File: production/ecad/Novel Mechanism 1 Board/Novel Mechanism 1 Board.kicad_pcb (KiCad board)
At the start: 2 copper layers, 39 parts, among them J1 Conn_01x02_Socket, J2 Conn_01x02_Socket, J3 Conn_01x02_Socket, J4 0532611271, U1 ADC081C021CIMM/NOPB, U2 ADC081C021CIMM/NOPB, U3 ADC081C021CIMM/NOPB

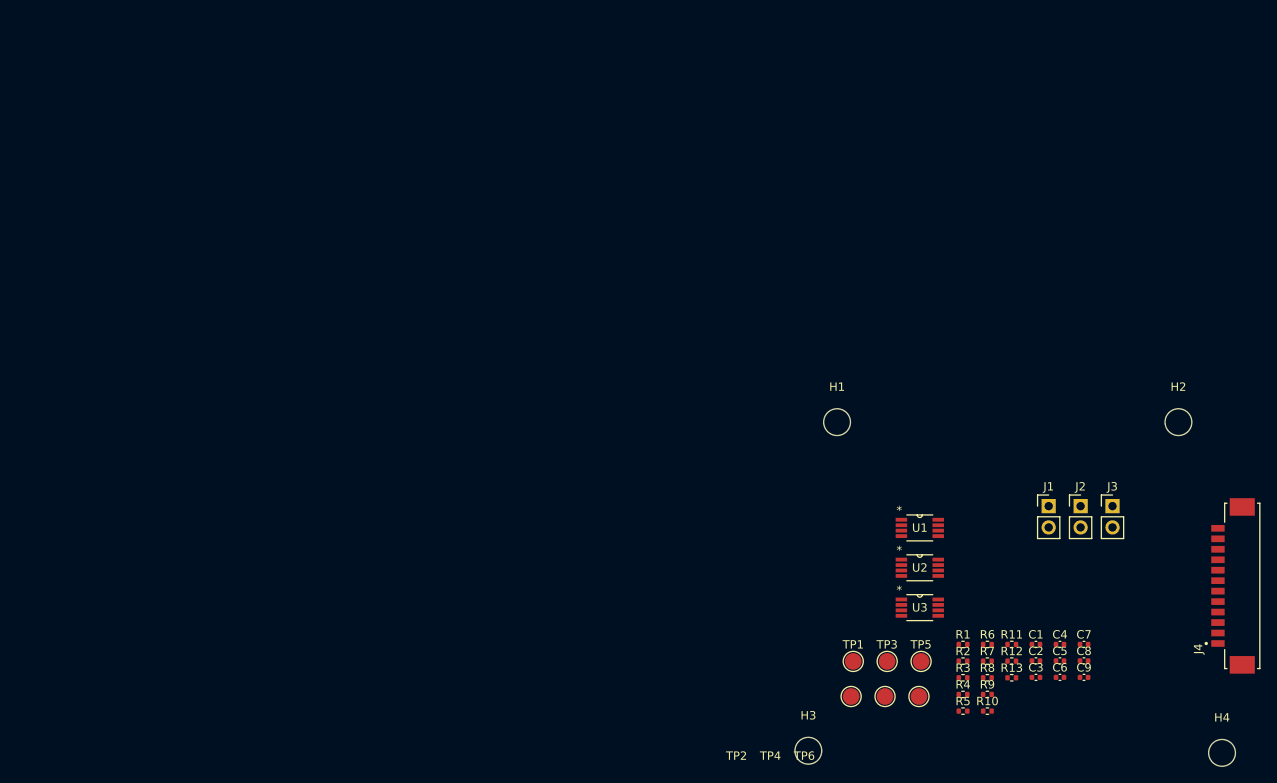
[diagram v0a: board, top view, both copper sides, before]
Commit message: layout
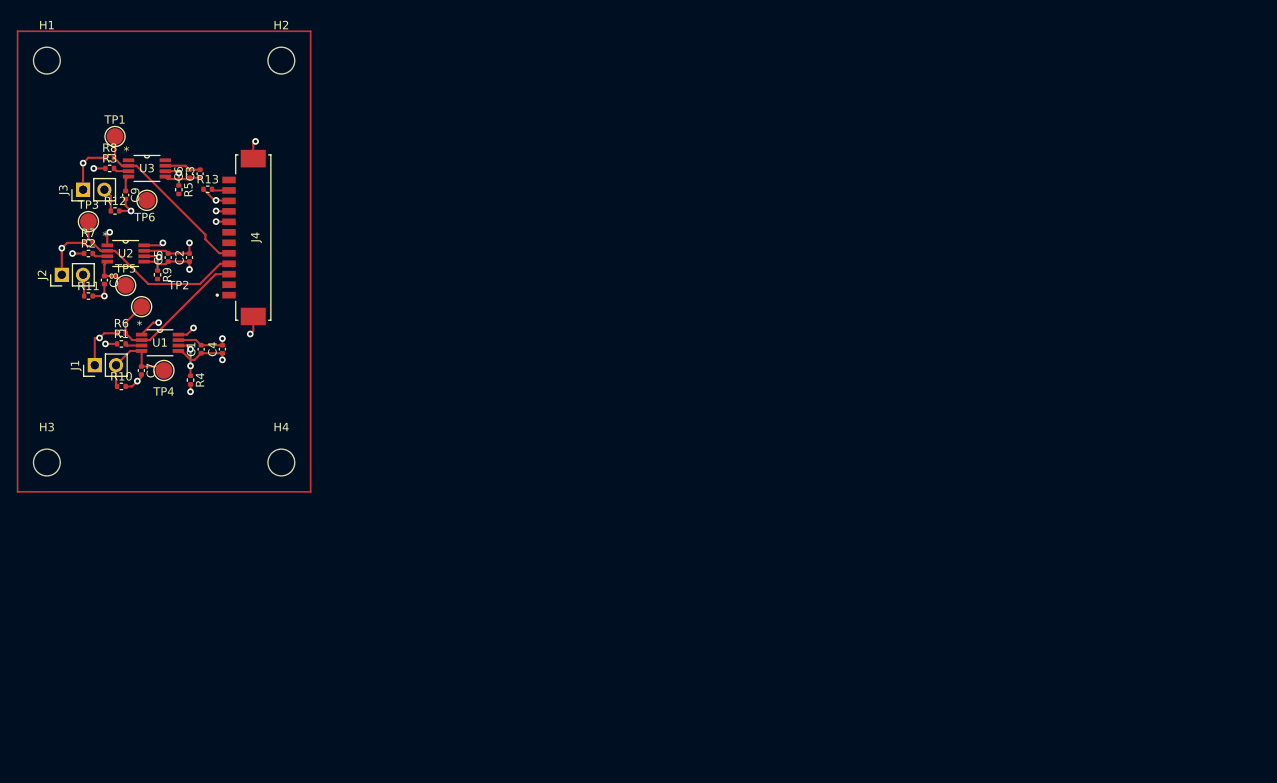
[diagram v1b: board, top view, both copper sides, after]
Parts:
- moved J3 128.6 mm to (27.4, 39.0), turned to 90 degrees
- moved C9 128.1 mm to (32.5, 39.7), turned to -90 degrees
- moved C8 125.5 mm to (30.0, 49.8), turned to -90 degrees
- moved J4 125.2 mm to (47.8, 44.8)
- moved J2 124.8 mm to (24.9, 49.2), turned to 90 degrees
- moved R8 121.8 mm to (30.6, 35.2)
- moved C6 120.1 mm to (40.1, 37.1), turned to 90 degrees
- moved R12 119.8 mm to (31.2, 41.6)
- moved R3 118.7 mm to (30.6, 36.5)
- moved R7 118.4 mm to (28.1, 45.4)
- moved R11 117.9 mm to (28.1, 51.7)
- moved H4 117.6 mm to (51.1, 71.6)
- moved C7 117.2 mm to (34.4, 60.6), turned to -90 degrees
- moved C5 116.9 mm to (37.6, 47.1), turned to 90 degrees
- moved C3 116.5 mm to (41.4, 37.1), turned to 90 degrees
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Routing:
- net GND: track 0.00 -> 37.8 mm, vias 0 -> 11
- net +3V3: track 0.00 -> 36.9 mm, vias 0 -> 5
- net INTERRUPT_F1: track 0.00 -> 22.1 mm
- net INTERRUPT_F2: track 0.00 -> 21.4 mm
- net INTERRUPT_LP: track 0.00 -> 19.9 mm
- net LIN_POT: track 0.00 -> 11.2 mm
- net FSR_1: track 0.00 -> 7.46 mm
- net SDA: track 0.00 -> 6.07 mm, vias 0 -> 3
- net SCL: track 0.00 -> 5.92 mm, vias 0 -> 3
- net Net-(U1-ADDR1): track 0.00 -> 4.80 mm, vias 0 -> 2
- net FSR_2: track 0.00 -> 4.72 mm
- net Net-(U2-ADDR1): track 0.00 -> 3.60 mm, vias 0 -> 1
- net Net-(U3-ADDR1): track 0.00 -> 3.28 mm, vias 0 -> 1
- net Net-(J4-Pad11): track 0.00 -> 2.09 mm
- net Net-(U1-ADDR0): track 0.00 -> 1.98 mm
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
